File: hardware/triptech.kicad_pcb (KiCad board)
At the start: 2 copper layers, 144.8 x 95.2 mm, 4 parts

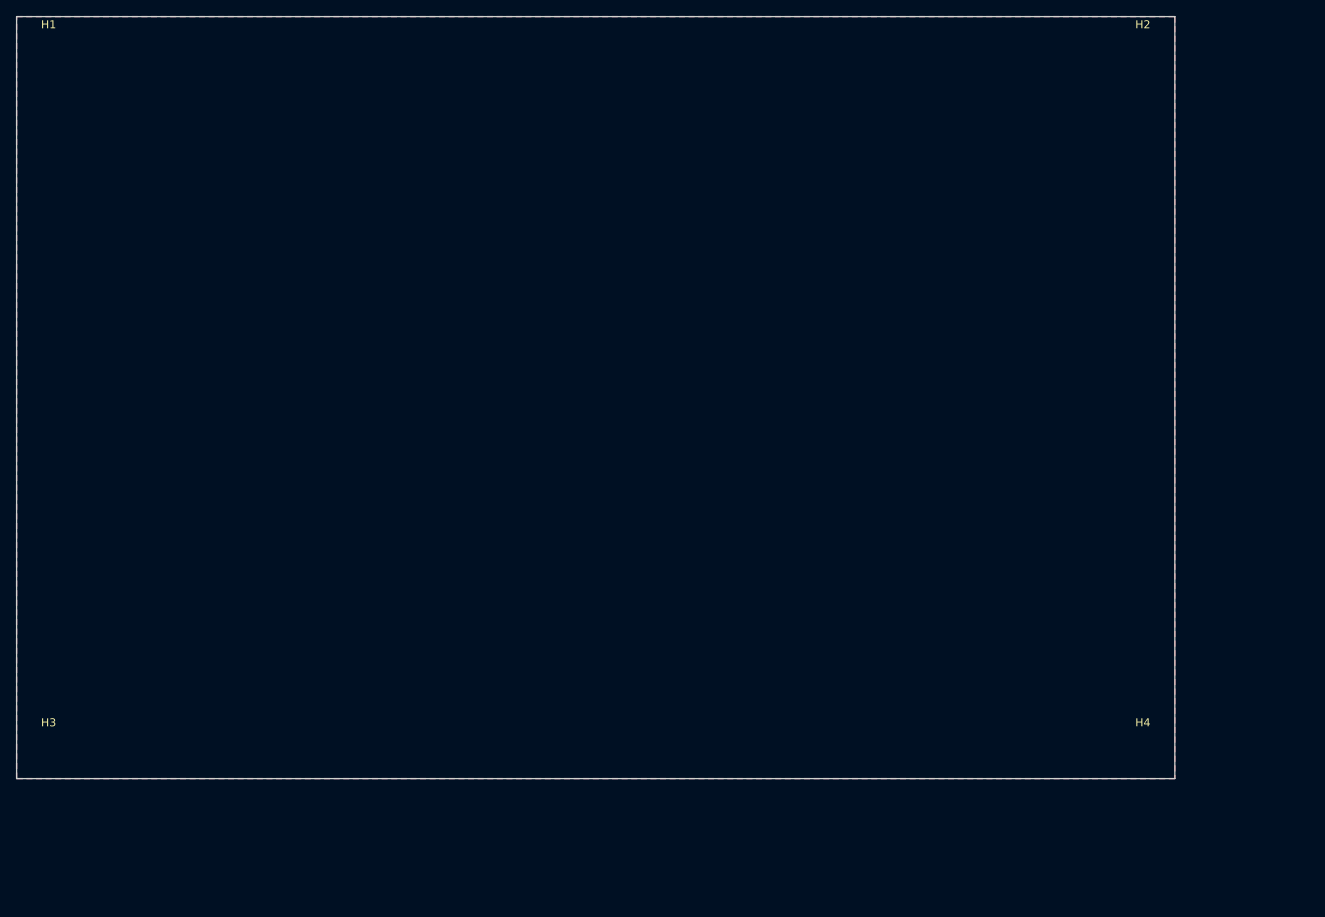
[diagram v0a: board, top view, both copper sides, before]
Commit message: WIP
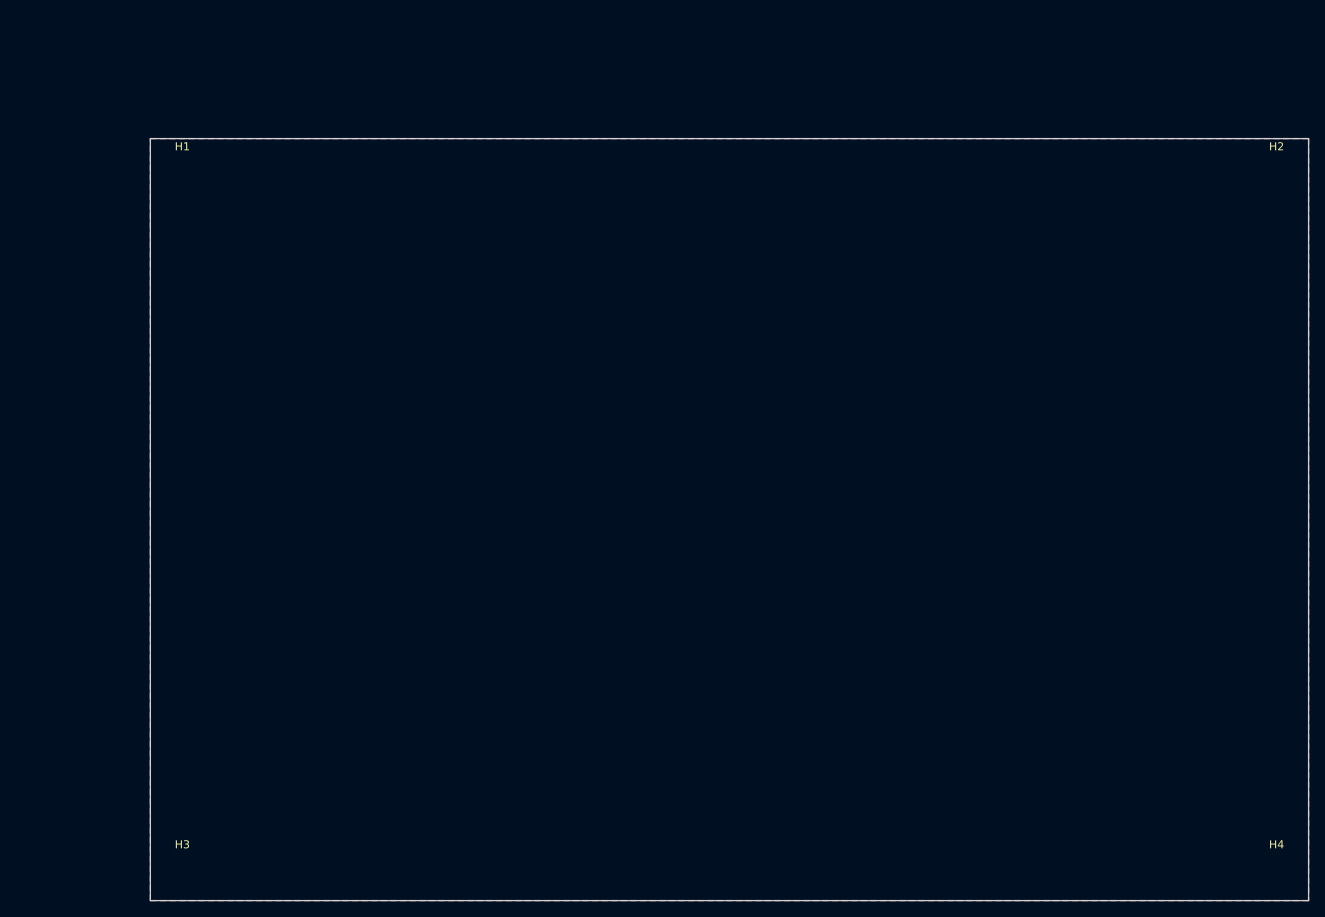
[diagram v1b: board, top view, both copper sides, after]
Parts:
- moved H1 22.6 mm to (20.7, 19.2)
- moved H2 22.6 mm to (157.5, 19.2)
- moved H3 22.6 mm to (20.7, 106.5)
- moved H4 22.6 mm to (157.5, 106.5)
